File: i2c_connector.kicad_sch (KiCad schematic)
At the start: 5 parts, among them J3 SM04B-SRSS-TB(LF)(SN)

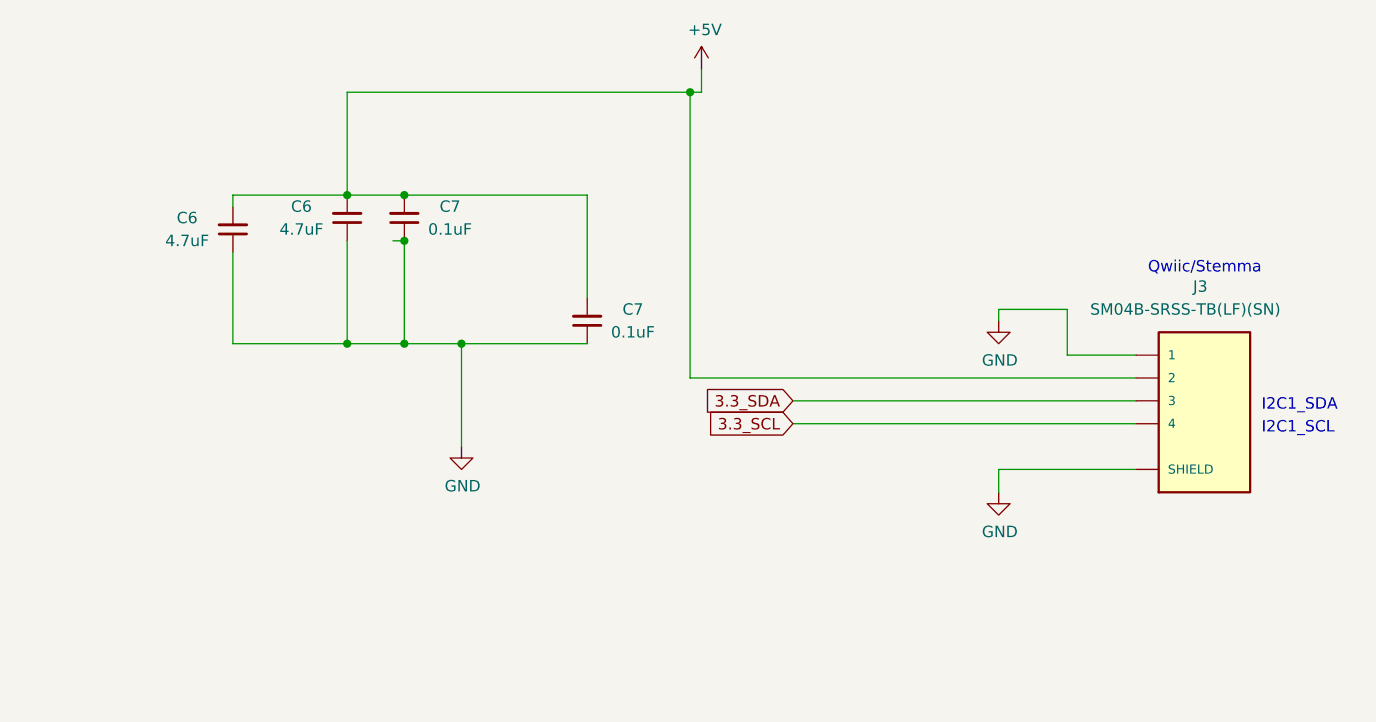
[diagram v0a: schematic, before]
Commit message: Fix connections
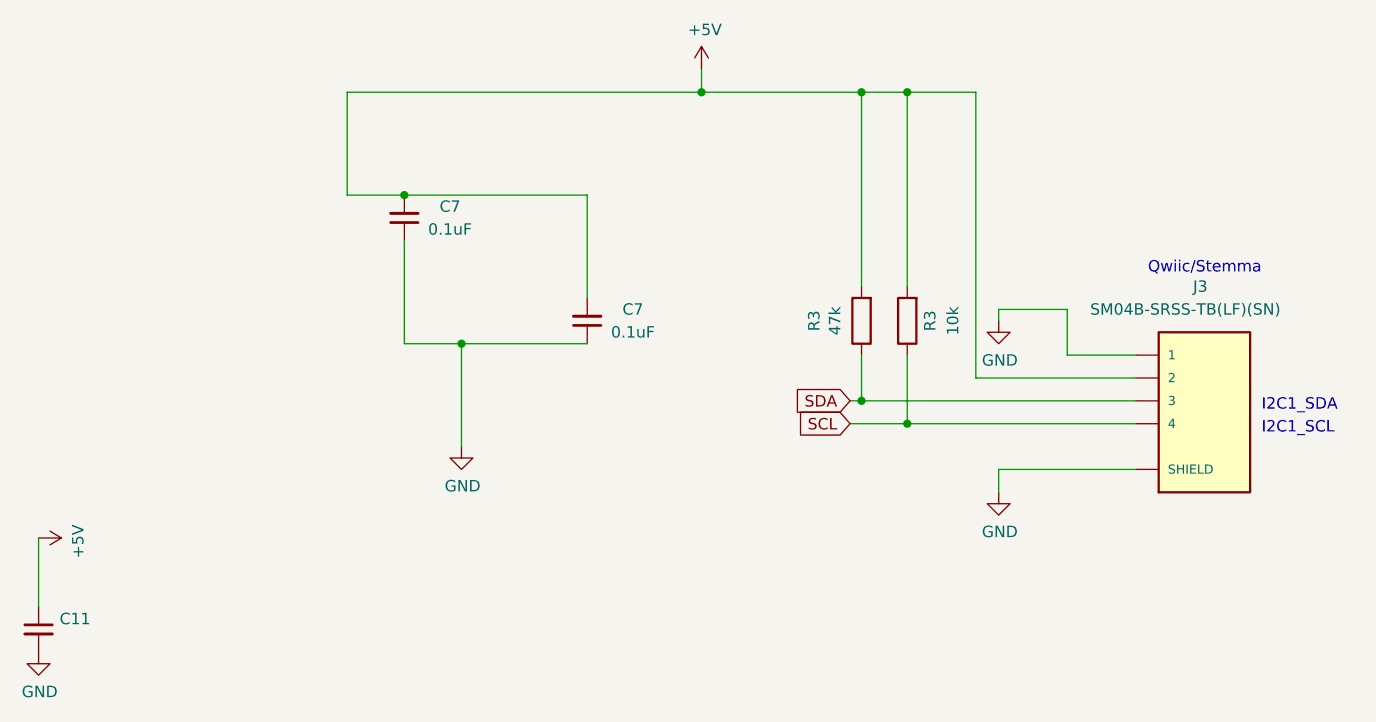
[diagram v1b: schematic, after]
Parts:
- removed C6 (x2): 4.7uF, Capacitor_SMD:C_0603_1608Metric, symbol Device:C_Small
- added C11: 10uF, Capacitor_SMD:C_0603_1608Metric, symbol Device:C_Small
- added R3: 10k, Resistor_SMD:R_0603_1608Metric, symbol Device:R
- added R3: 47k, Resistor_SMD:R_0603_1608Metric, symbol Device:R
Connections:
- net +5V: now also C11.1, R3.2, R3.2
- net GND: now also C11.2
- net 3.3_SCL renamed SCL
- net SCL: now also R3.1
- net 3.3_SDA renamed SDA
- net SDA: now also R3.1
